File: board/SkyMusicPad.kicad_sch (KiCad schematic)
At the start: 36 parts, among them SW1 Cherry, SW10 Cherry, SW11 Cherry, SW12 Cherry, SW13 Cherry, SW14 Cherry, SW15 Cherry, SW16 RotaryEncoder_Switch, SW2 Cherry, SW3 Cherry, SW4 Cherry, SW5 Cherry, SW6 Cherry, SW7 Cherry, SW8 Cherry, SW9 Cherry, U1 ESP32-S3-Zero

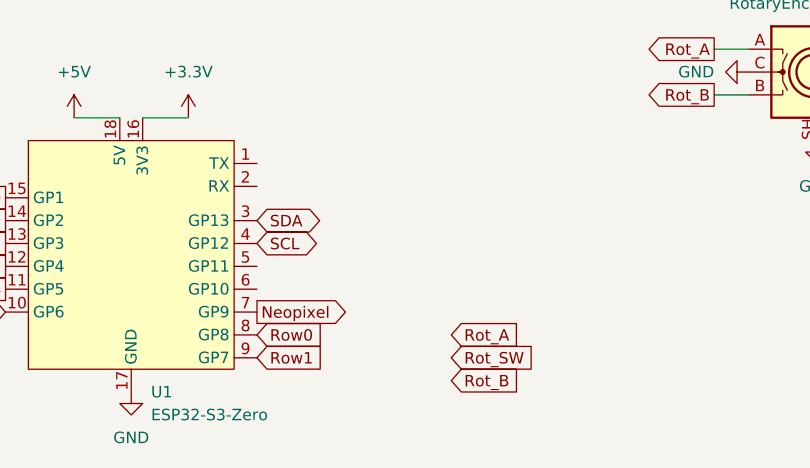
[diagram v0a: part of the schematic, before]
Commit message: Code and PCB updates
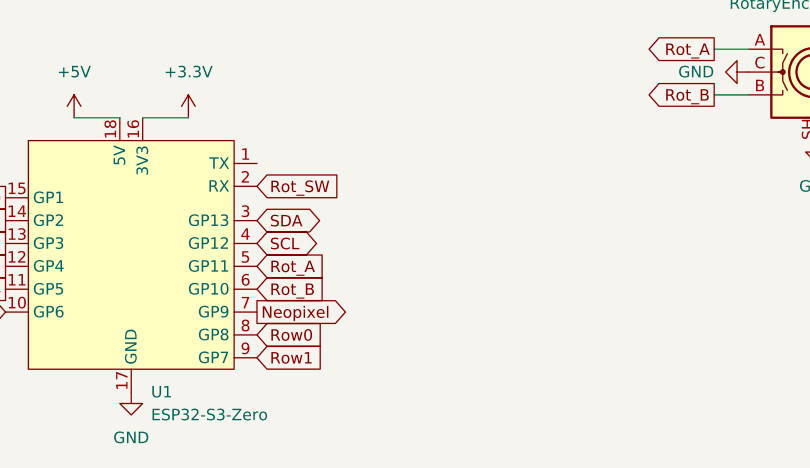
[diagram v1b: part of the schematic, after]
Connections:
- net Rot_A: now also U1.5 (GP11)
- net Rot_B: now also U1.6 (GP10)
- net Rot_SW: now also U1.2 (RX)
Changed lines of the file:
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@@
 	(global_label "Rot_B"
 		(shape input)
-		(at 101.6 153.67 0)
-		(fields_autoplaced yes)
-		(effects
-			(font
-				(size 1.27 1.27)
-			)
-			(justify left)
-		)
-		(property "Intersheetrefs" "${INTERSHEET_REFS}"
-			(at 109.9675 153.67 0)
+		(at 80.01 143.51 0)
+		(fields_autoplaced yes)
+		(effects
+			(font
+				(size 1.27 1.27)
+			)
+			(justify left)
+		)
+		(property "Intersheetrefs" "${INTERSHEET_REFS}"
+			(at 88.3775 143.51 0)
 			(effects
 				(font
@@
 	(global_label "Rot_SW"
 		(shape input)
-		(at 101.6 151.13 0)
-		(fields_autoplaced yes)
-		(effects
-			(font
-				(size 1.27 1.27)
-			)
-			(justify left)
-		)
-		(property "Intersheetrefs" "${INTERSHEET_REFS}"
-			(at 111.3584 151.13 0)
+		(at 80.01 132.08 0)
+		(fields_autoplaced yes)
+		(effects
+			(font
+				(size 1.27 1.27)
+			)
+			(justify left)
+		)
+		(property "Intersheetrefs" "${INTERSHEET_REFS}"
+			(at 89.7684 132.08 0)
 			(effects
 				(font
@@
 	(global_label "Rot_A"
 		(shape input)
-		(at 101.6 148.59 0)
-		(fields_autoplaced yes)
-		(effects
-			(font
-				(size 1.27 1.27)
-			)
-			(justify left)
-		)
-		(property "Intersheetrefs" "${INTERSHEET_REFS}"
-			(at 109.7861 148.59 0)
-			(effects
-				(font
+		(at 80.01 140.97 0)
+		(fields_autoplaced yes)
+		(effects
+			(font
+				(size 1.27 1.27)
+			)
+			(justify left)
+		)
+		(property "Intersheetrefs" "${INTERSHEET_REFS}"
+			(at 88.1961 140.97 0)
+			(effects
+				(font

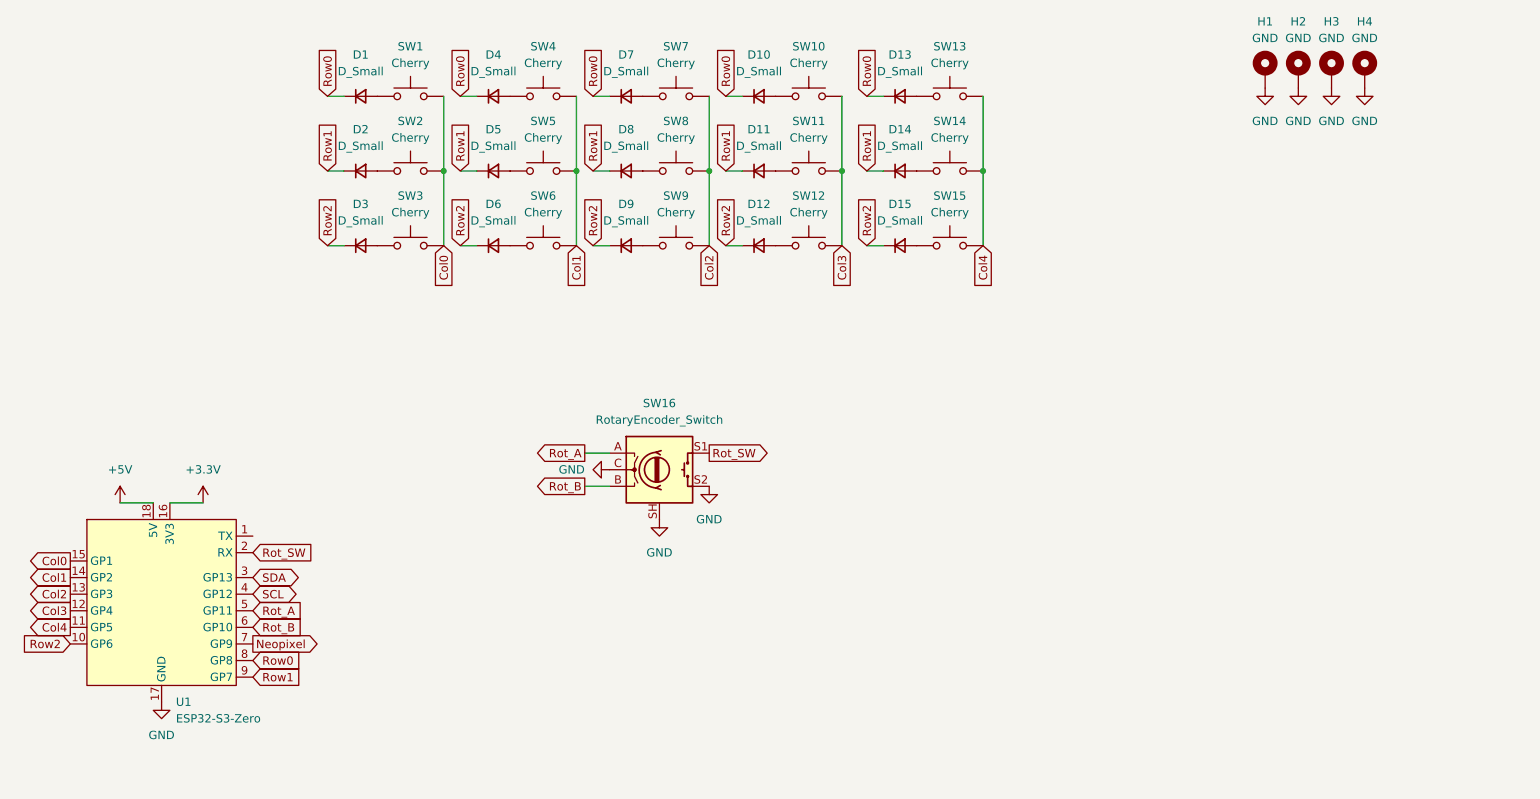
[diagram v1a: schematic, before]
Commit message: Further board and code development.
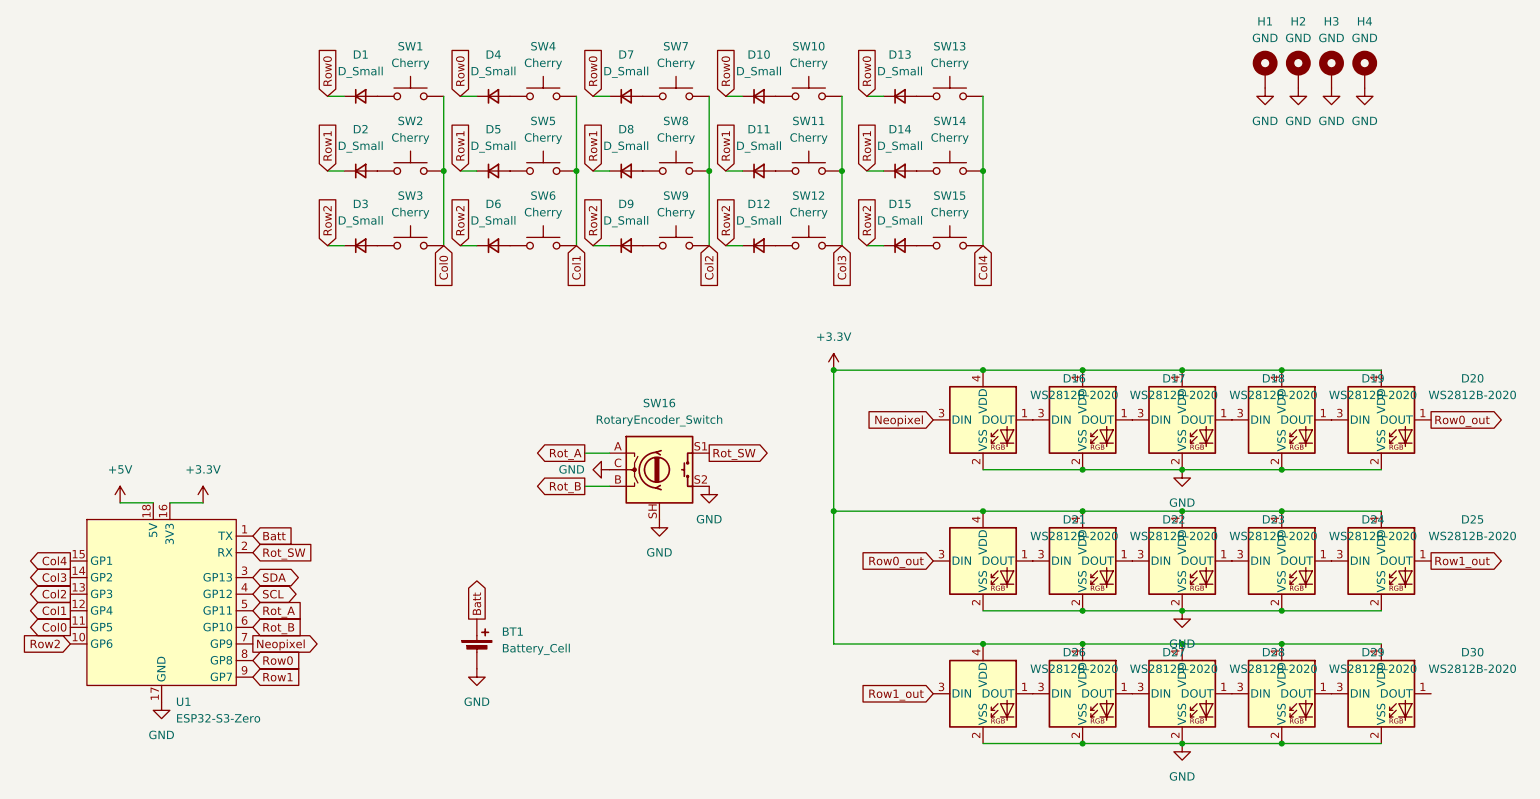
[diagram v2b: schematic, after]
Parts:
- added BT1: Battery_Cell, symbol Device:Battery_Cell
- added D16, D17, D18, D19, D20, D21, D22, D23, D24, D25, D26, D27, D28, D29, D30: WS2812B-2020, LED_SMD:LED_WS2812B-2020_PLCC4_2.0x2.0mm, symbol LED:WS2812B-2020
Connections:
- net +3.3V: now also D16.4 (VDD), D17.4 (VDD), D18.4 (VDD), D19.4 (VDD), D20.4 (VDD), D21.4 (VDD), D22.4 (VDD), D23.4 (VDD), D24.4 (VDD), D25.4 (VDD), D26.4 (VDD), D27.4 (VDD), D28.4 (VDD), D29.4 (VDD), D30.4 (VDD)
- net Col0: now also U1.11 (GP5); no longer U1.15 (GP1)
- net Col1: now also U1.12 (GP4); no longer U1.14 (GP2)
- net Col3: now also U1.14 (GP2); no longer U1.12 (GP4)
- net Col4: now also U1.15 (GP1); no longer U1.11 (GP5)
- net GND: now also BT1.2 (-), D16.2 (VSS), D17.2 (VSS), D18.2 (VSS), D19.2 (VSS), D20.2 (VSS), D21.2 (VSS), D22.2 (VSS), D23.2 (VSS), D24.2 (VSS), D25.2 (VSS), D26.2 (VSS), D27.2 (VSS), D28.2 (VSS), D29.2 (VSS), D30.2 (VSS)
- net Neopixel: now also D16.3 (DIN)
- net Batt: now reaches U1.1 (TX)
- net Batt: now also BT1.1 (+)
- new net: D16.1 (DOUT), D17.3 (DIN)
- new net: D27.1 (DOUT), D28.3 (DIN)
- new net: D26.1 (DOUT), D27.3 (DIN)
- new net: D18.1 (DOUT), D19.3 (DIN)
- new net: D17.1 (DOUT), D18.3 (DIN)
- new net: D22.1 (DOUT), D23.3 (DIN)
- new net: D21.1 (DOUT), D22.3 (DIN)
- new net: D29.1 (DOUT), D30.3 (DIN)
- new net: D24.1 (DOUT), D25.3 (DIN)
- new net: D23.1 (DOUT), D24.3 (DIN)
- new net: D28.1 (DOUT), D29.3 (DIN)
- new net: D19.1 (DOUT), D20.3 (DIN)
- new net Row0_out: D20.1 (DOUT), D21.3 (DIN)
- new net Row1_out: D25.1 (DOUT), D26.3 (DIN)
